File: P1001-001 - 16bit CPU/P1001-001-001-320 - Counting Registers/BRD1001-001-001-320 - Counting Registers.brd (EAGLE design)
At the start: 200 x 48 mm, 19 parts, among them IC1 74HC192D, IC12 74AC245DW, IC2 74HC192D, IC27 MEGA8535-A, IC3 74HC192D, IC4 74HC192D, IC7 74AC245DW, J1 22-27-2041-04

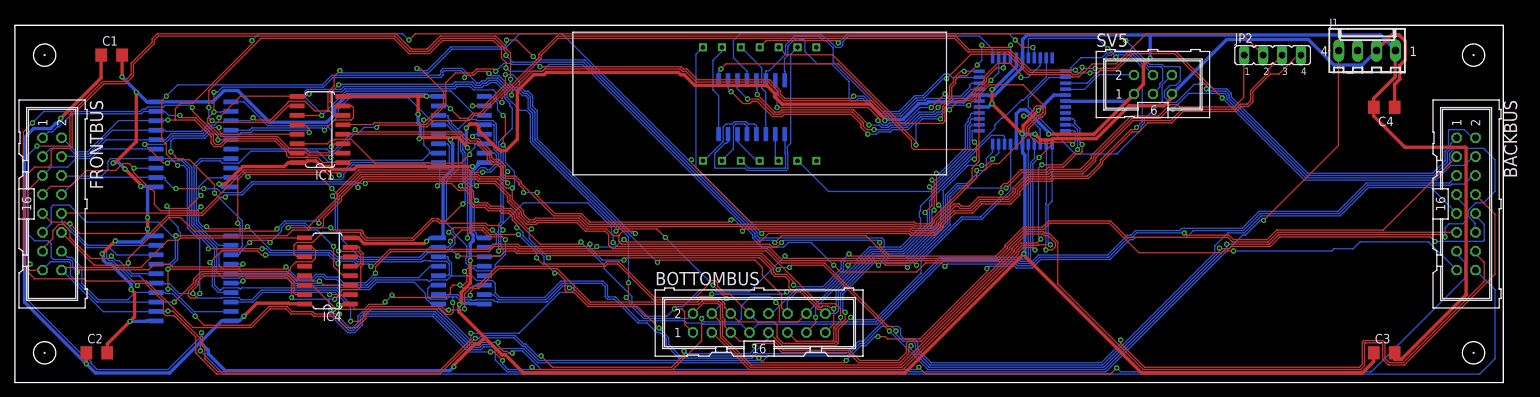
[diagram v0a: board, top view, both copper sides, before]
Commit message: Add the prototype stuff
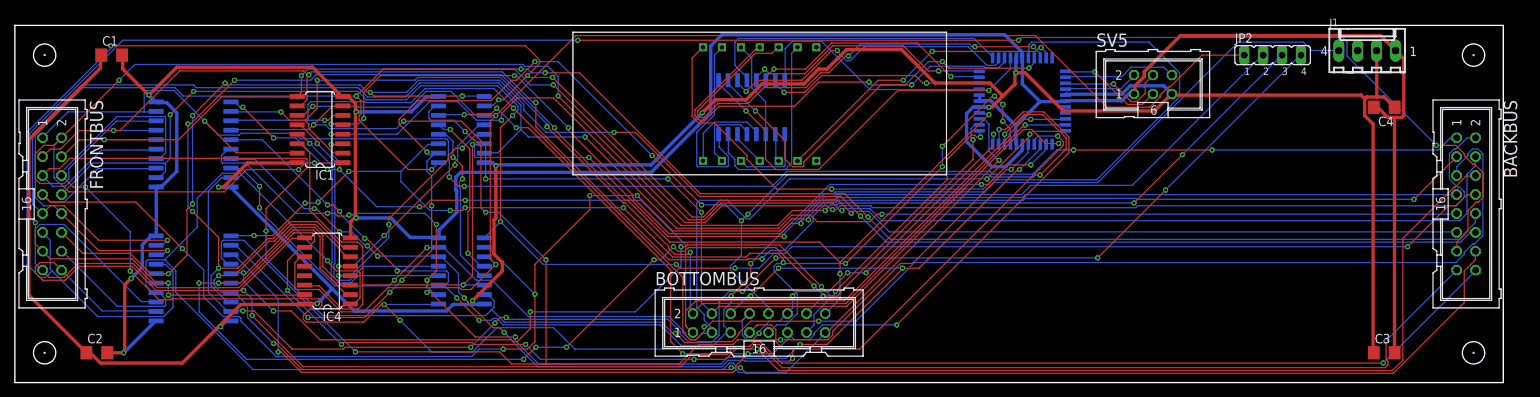
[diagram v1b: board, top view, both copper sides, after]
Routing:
- net SIGNAL4: track 236.4 -> 141.4 mm, vias 6 -> 10
- net SIGNAL12: track 228.6 -> 156.8 mm, vias 8 -> 7
- net VCC: track 444.0 -> 379.0 mm, vias 14 -> 8
- net SIGNAL2: track 229.0 -> 165.5 mm, vias 6 -> 4
- net SIGNAL11: track 237.3 -> 175.7 mm, vias 8 -> 9
- net SIGNAL5: track 229.4 -> 171.7 mm, vias 5 -> 11
- net GND: track 406.7 -> 350.2 mm, vias 21 -> 5
- net CLEAR: track 253.3 -> 207.4 mm, vias 9 -> 4
- net BUS1: track 246.4 -> 291.8 mm, vias 4 -> 5
- net BUS12: track 233.4 -> 278.4 mm
- net !REG_IN: track 244.2 -> 200.4 mm, vias 5 -> 3
- net SIGNAL10: track 171.2 -> 214.8 mm
- net SIGNAL15: track 143.8 -> 187.5 mm, vias 8 -> 7
- net SIGNAL1: track 196.6 -> 153.4 mm, vias 9 -> 5
- net BUS5: track 224.4 -> 266.0 mm, vias 4 -> 5
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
